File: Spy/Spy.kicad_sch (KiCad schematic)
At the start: 11 parts, among them J1 Screw_Terminal_01x02, J2 Screw_Terminal_01x02, U1 ESP32-DevKitC, U2 GP2Y0A21YK0F, U3 GP2Y0A21YK0F, U4 SEN-12787, U5 L298N, U6 QTR-8A, U7 3190

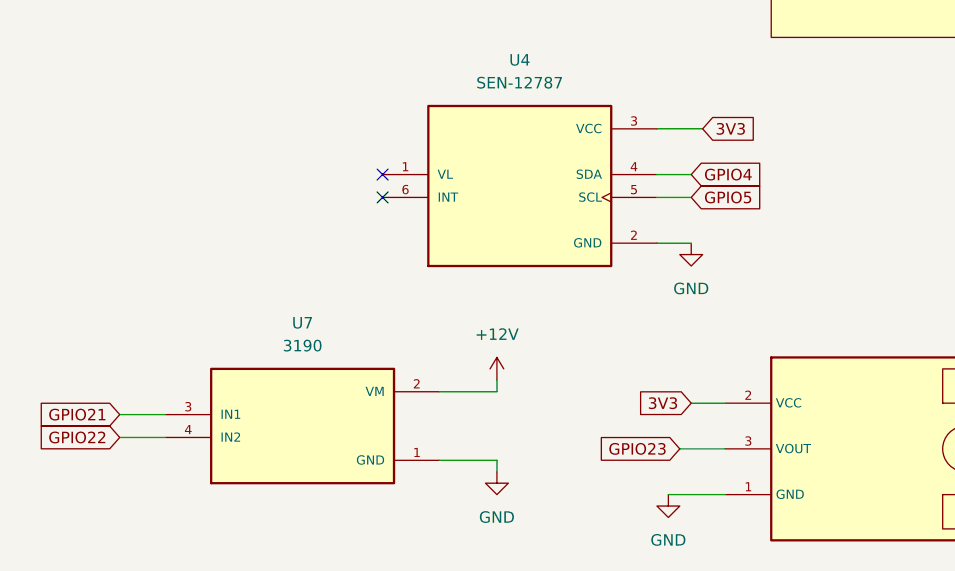
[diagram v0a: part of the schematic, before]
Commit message: rewired some stuff
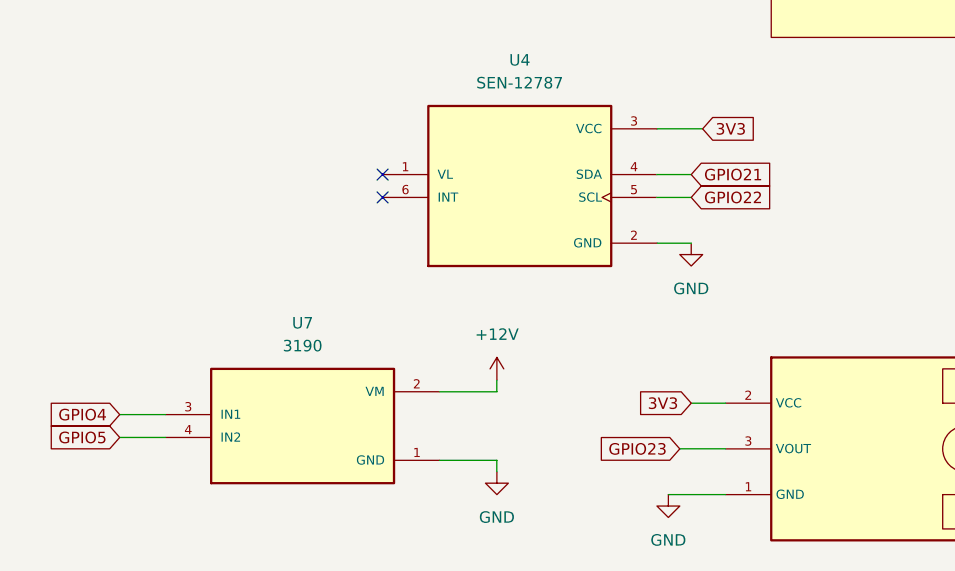
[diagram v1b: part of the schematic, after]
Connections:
- net GPIO21: now also U4.4 (SDA); no longer U7.3 (IN1)
- net GPIO22: now also U4.5 (SCL); no longer U7.4 (IN2)
- net GPIO4: now also U7.3 (IN1); no longer U4.4 (SDA)
- net GPIO5: now also U7.4 (IN2); no longer U4.5 (SCL)
